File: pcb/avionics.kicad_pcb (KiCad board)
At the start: 2 copper layers, 100 x 48 mm, 108 parts, among them IC101 STM32F405VGT, IC102 ADP3335, IC201 MAX-7Q, IC701 ADXL345, IC702 L3G4200D, IC703 MS5611-01BA03, IC704 HMC5883L, P101 CONN_01X02, P102 CONN_01X04, P103 SWD, P201 SMA, P202 SMA, P501 CONN_01X02, P502 CONN_01X02, P503 CONN_01X02, P504 CONN_01X02, Q501 IRF7910, Q502 FDN304P, Q503 FDN304P, Q504 IRF7910, Q505 FDN304P, Q506 FDN304P, Q601 IRF7910, U202 RFM69W, U401 MICROSD_HOLDER, X101 8M

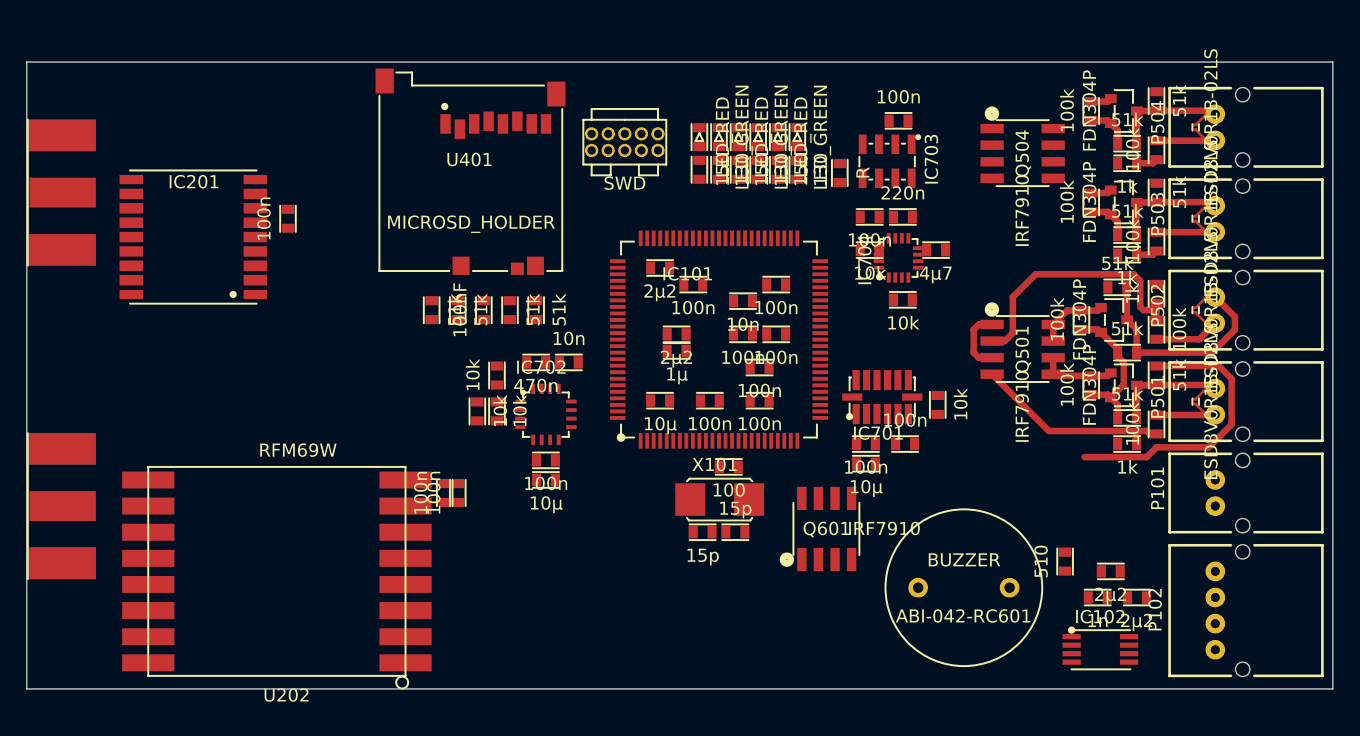
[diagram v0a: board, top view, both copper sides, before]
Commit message: continue pyro routing
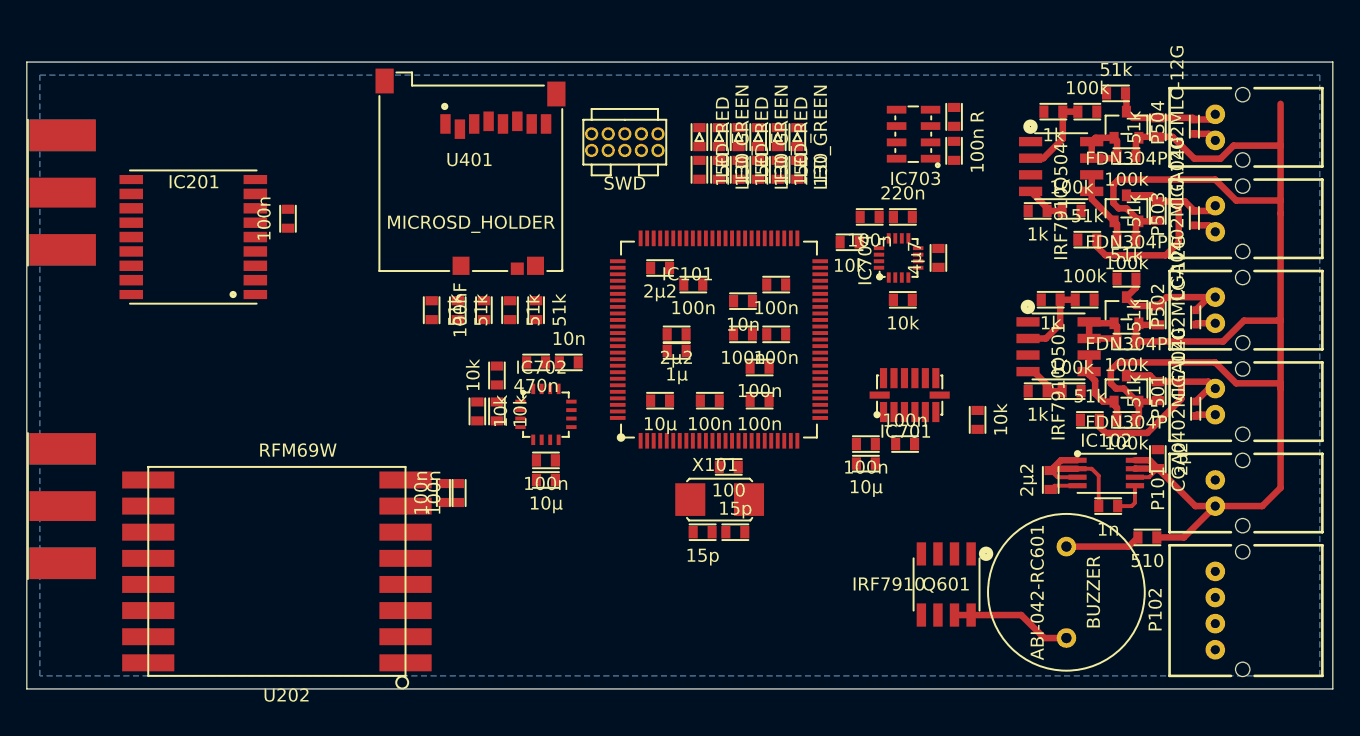
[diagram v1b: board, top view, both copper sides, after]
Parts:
- D501, D502, D503, D504: value ESD8V0R1B-02LS -> CGA0402MLC-12G; footprint avionics14:TSSLP-2-1 -> avionics14:R0402
- moved IC102 13.5 mm to (168.4, 71.5)
- moved C117 11.2 mm to (166.4, 73.0), turned to 270 degrees
- moved Q601 10.1 mm to (158.4, 81.0), turned to 180 degrees
- moved R706 9.75 mm to (159.0, 45.2)
- moved C115 9.32 mm to (174.6, 71.4), turned to 90 degrees
- moved R511 8.11 mm to (166.4, 59.2), turned to 0 degrees
- moved R501 7.96 mm to (165.4, 66.2)
- moved ABI-042-RC601 7.86 mm to (167.6, 81.6), turned to 270 degrees
- moved R502 7.63 mm to (165.4, 52.4)
- moved C116 7.05 mm to (170.8, 75.0)
- moved R503 6.98 mm to (168.0, 66.2), turned to 180 degrees
- moved R504 6.91 mm to (168.0, 52.4), turned to 180 degrees
- moved R512 6.89 mm to (166.6, 44.8)
- moved R607 6.57 mm to (173.8, 77.4), turned to 0 degrees
- moved R510 6.41 mm to (169.2, 54.6), turned to 180 degrees
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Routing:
- net +BATT: track 17.8 -> 121.4 mm
- net GND: track 30.8 -> 8.87 mm
- net /Datalogging & Pyros/~PY1_CHK: track 21.9 -> 0.00 mm
- net Net-(Q501-Pad2): track 19.9 -> 5.94 mm
- net Net-(Q501-Pad4): track 16.0 -> 3.51 mm
- net +3V3: track 0.00 -> 10.9 mm
- net Net-(ABI-042-RC601-Pad2): track 0.00 -> 9.29 mm
- net Net-(D501-Pad1): track 10.5 -> 18.9 mm
- net Net-(D502-Pad1): track 18.9 -> 11.0 mm
- net Net-(D503-Pad1): track 10.5 -> 18.1 mm
- net Net-(ABI-042-RC601-Pad1): track 0.00 -> 5.76 mm
- net Net-(Q504-Pad7): track 1.59 -> 6.60 mm
- net Net-(Q504-Pad2): track 1.64 -> 6.31 mm
- net Net-(Q503-Pad1): track 1.59 -> 5.77 mm
- net Net-(C116-Pad2): track 0.00 -> 2.74 mm
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- added copper zone on B.Cu, net GND
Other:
- net class Default: via_dia 1.4 -> 1; via_drill 0.8 -> 0.6
- rule trace_min: 0.15 -> 0.2
- rule via_min_size: 1.2 -> 1
